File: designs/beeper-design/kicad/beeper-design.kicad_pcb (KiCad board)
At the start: 4 copper layers, 27.5 x 19.1 mm, 209 parts

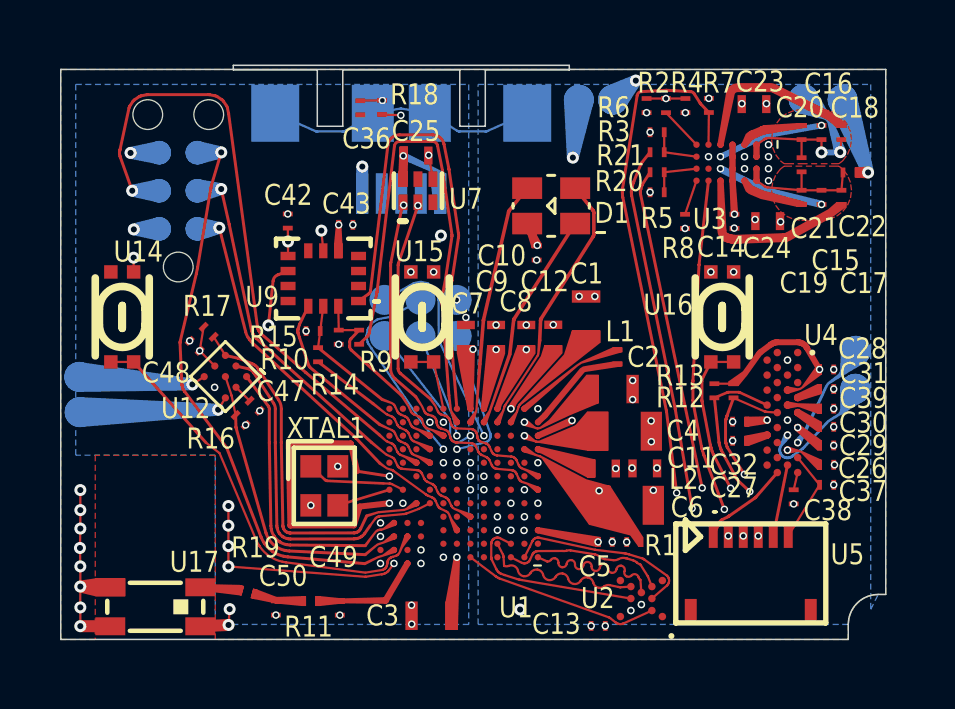
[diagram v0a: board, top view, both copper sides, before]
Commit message: latest fully routed version
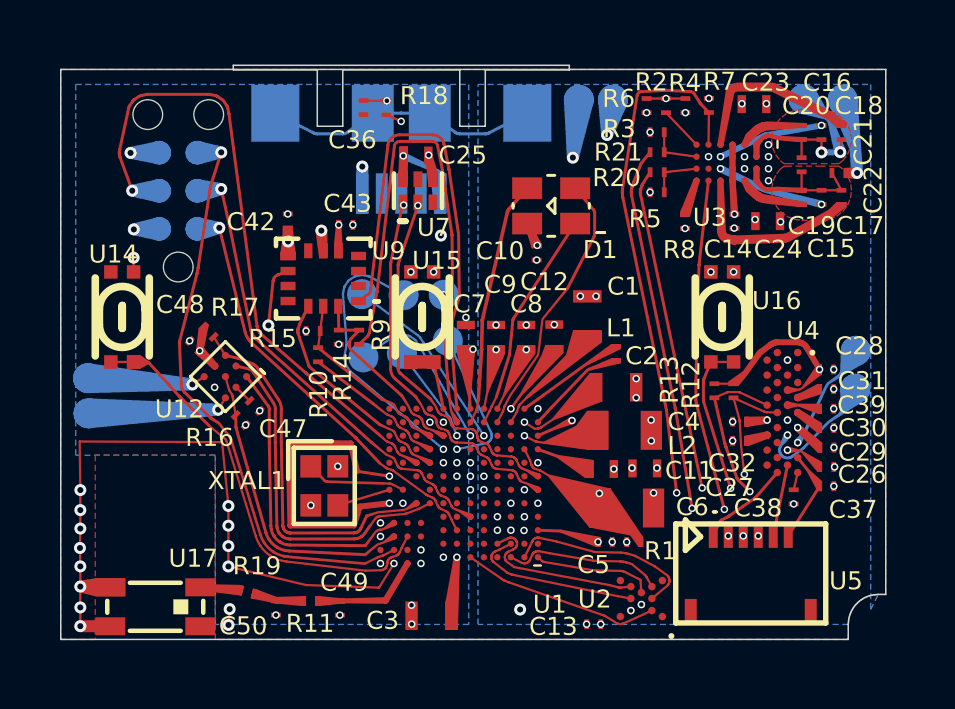
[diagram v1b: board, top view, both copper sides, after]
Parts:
- removed the ? at (143.1, 109.2)
- removed the ? at (149.4, 102.4)
- removed the ? at (141.3, 111.2)
- removed the ? at (149.9, 110.8)
- removed the ? at (151.5, 109.2)
- removed the ? at (150.7, 110.8)
- removed the ? at (149.7, 102.7)
- removed the ? at (152.1, 100.6)
- removed the ? at (148.7, 102.7)
- removed the ? at (136.6, 110.4)
- removed the ? at (148.6, 100.8)
- removed the ? at (140.2, 108.8)
- removed the C18 at (151.8, 100.6)
- removed the C2 at (144.1, 109.2)
- removed the R16 at (131.7, 110.2)
- removed the TP12 at (144.2, 99.5)
- added ?: , beeper-design:dummy114, F.Cu at (137.8, 108.2)
- added ?: , beeper-design:dummy115, F.Cu at (128.7, 102.5)
- added ?: , beeper-design:dummy117, F.Cu at (137.4, 111.5)
- added ?: , beeper-design:dummy116, F.Cu at (136.5, 110.8)
- added C28: 1u, beeper-design:Pkg0201_12, F.Cu at (151.3, 108.5)
- added C37: 1u, beeper-design:Pkg0201_10, F.Cu at (151.3, 112.4)
- added C43: 100n, beeper-design:Pkg0201_26, F.Cu at (135.3, 103.7)
- added C49: 1p, beeper-design:Pkg0201_13, F.Cu at (135.1, 116.5)
- added L2: 1u, beeper-design:Pkg0402_5, F.Cu at (143.8, 111.8)
- added R4: 20K, beeper-design:Pkg0201_34, F.Cu at (146.6, 99.7)
- added R5: 10K, beeper-design:Pkg0201_44, F.Cu at (145.6, 102.6)
- added R9: 0R, beeper-design:Pkg0201_8, F.Cu at (135.7, 107.4)
- added TP4: ~, beeper-design:SMD_TESTPT, B.Cu at (152.3, 107.9)
- added TP6: ~, beeper-design:SMD_TESTPT, B.Cu at (137.2, 106.0)
- added TP8: ~, beeper-design:SMD_TESTPT, B.Cu at (138.7, 107.5)
- added TP9: ~, beeper-design:SMD_TESTPT, B.Cu at (135.8, 108.1)
- added U15: ~, beeper-design:LP_1, F.Cu at (137.8, 106.8)
- added U16: ~, beeper-design:LP_1, F.Cu at (147.8, 106.8)
- added U17: ~, beeper-design:Pkg_2450AT18D0100_STD_R_1, F.Cu at (128.9, 116.4)
- added U2: ~, beeper-design:WLCSP_12, F.Cu at (145.1, 116.1)
- ?: renamed from U15; value ~ -> (none); footprint beeper-design:LP_2 -> beeper-design:dummy1
- ?: renamed from TP9; value ~ -> (none); footprint beeper-design:SMD_TESTPT -> beeper-design:dummy31; moved to F.Cu
- ?: renamed from R9; value 0R -> (none); footprint beeper-design:Pkg0201_32 -> beeper-design:dummy89
- ?: renamed from L2; value 1u -> (none); footprint beeper-design:Pkg0402_1 -> beeper-design:dummy17
- ?: renamed from C49; value 1p -> (none); footprint beeper-design:Pkg0201_34 -> beeper-design:dummy112
- ?: renamed from U16; value ~ -> (none); footprint beeper-design:LP_2 -> beeper-design:dummy64
- ?: renamed from R4; value 20K -> (none); footprint beeper-design:Pkg0201_18 -> beeper-design:dummy38
- ?: renamed from TP6; value ~ -> (none); footprint beeper-design:SMD_TESTPT -> beeper-design:dummy26; moved to F.Cu
- ?: renamed from C28; value 1u -> (none); footprint beeper-design:Pkg0201_19 -> beeper-design:dummy80
- ?: renamed from TP8; value ~ -> (none); footprint beeper-design:SMD_TESTPT -> beeper-design:dummy45; moved to F.Cu
- ?: renamed from U17; value ~ -> (none); footprint beeper-design:Pkg_2450AT18D0100_STD_R_1 -> beeper-design:dummy98
- ?: renamed from U2; value ~ -> (none); footprint beeper-design:WLCSP_12 -> beeper-design:dummy52
- C1: footprint beeper-design:Pkg0603_2 -> beeper-design:Pkg0603_1
- C10: footprint beeper-design:Pkg0201_8 -> beeper-design:Pkg0201_38
- C11: footprint beeper-design:Pkg0402_4 -> beeper-design:Pkg0402_7
- C12: footprint beeper-design:Pkg0402_3 -> beeper-design:Pkg0402
- C13: footprint beeper-design:Pkg0201_10 -> beeper-design:Pkg0201
- C14: footprint beeper-design:Pkg0201_1 -> beeper-design:Pkg0201_45
- C15: footprint beeper-design:Pkg0201_4 -> beeper-design:Pkg0201_42
- C16: footprint beeper-design:Pkg0201_11 -> beeper-design:Pkg0201_4
- C17: footprint beeper-design:Pkg0201_17 -> beeper-design:Pkg0201_18
- C18: renamed from C43; value 100n -> 22n; footprint beeper-design:Pkg0201_22 -> beeper-design:Pkg0201_30
- C19: renamed from TP4; value ~ -> 10n; footprint beeper-design:SMD_TESTPT -> beeper-design:Pkg0201_41; moved to F.Cu
- C2: renamed from R5; value 10K -> 22u; footprint beeper-design:Pkg0201_26 -> beeper-design:Pkg0603_2
- C20: renamed from C19; footprint beeper-design:Pkg0201_31 -> beeper-design:Pkg0201_3
- C21: footprint beeper-design:Pkg0201_46 -> beeper-design:Pkg0201_16
- C22: footprint beeper-design:Pkg0201_3 -> beeper-design:Pkg0201_28
- C23: footprint beeper-design:Pkg0402_2 -> beeper-design:Pkg0402_8
- C24: footprint beeper-design:Pkg0402_5 -> beeper-design:Pkg0402_1
- C25: footprint beeper-design:Pkg0402_6 -> beeper-design:Pkg0402_3
- C26: footprint beeper-design:Pkg0201_24 -> beeper-design:Pkg0201_7
- C27: footprint beeper-design:Pkg0201_27 -> beeper-design:Pkg0201_24
- C29: footprint beeper-design:Pkg0201_42 -> beeper-design:Pkg0201_46
- C3: footprint beeper-design:Pkg0603_1 -> beeper-design:Pkg0603
- C30: footprint beeper-design:Pkg0201_12 -> beeper-design:Pkg0201_33
- C31: footprint beeper-design:Pkg0201_16 -> beeper-design:Pkg0201_43
- C36: footprint beeper-design:Pkg0201_36 -> beeper-design:Pkg0201_2
- C38: footprint beeper-design:Pkg0201_5 -> beeper-design:Pkg0201_21
- C39: footprint beeper-design:Pkg0201_30 -> beeper-design:Pkg0201_20
- C42: footprint beeper-design:Pkg0201_15 -> beeper-design:Pkg0201_14
- C47: footprint beeper-design:Pkg0201_7 -> beeper-design:Pkg0201_27
- C48: footprint beeper-design:Pkg0201_14 -> beeper-design:Pkg0201_37
- C5: footprint beeper-design:Pkg0201_20 -> beeper-design:Pkg0201_29
- C50: footprint beeper-design:Pkg0201_44 -> beeper-design:Pkg0201_32
- C7: footprint beeper-design:Pkg0402_7 -> beeper-design:Pkg0402_2
- C8: footprint beeper-design:Pkg0402_8 -> beeper-design:Pkg0402_4
- C9: footprint beeper-design:Pkg0402 -> beeper-design:Pkg0402_6
- D1: footprint beeper-design:LP_5 -> beeper-design:LP_4
- L1: footprint beeper-design:Pkg0201_2 -> beeper-design:Pkg0201_11
- R1: footprint beeper-design:Pkg0201_43 -> beeper-design:Pkg0201_47
- R10: footprint beeper-design:Pkg0201_38 -> beeper-design:Pkg0201_17
- R11: footprint beeper-design:Pkg0201_39 -> beeper-design:Pkg0201_22
- R12, R13: footprint beeper-design:Pkg0201_9 -> beeper-design:Pkg0201_1
- R14, R15: footprint beeper-design:Pkg0201_23 -> beeper-design:Pkg0201_36
- R16: renamed from C20; value 10n -> 8K2; footprint beeper-design:Pkg0201_40 -> beeper-design:Pkg0201_5
- R17: footprint beeper-design:Pkg0201_21 -> beeper-design:Pkg0201_5
- R18: footprint beeper-design:Pkg0201_28 -> beeper-design:Pkg0201_40
- R19: footprint beeper-design:Pkg0201 -> beeper-design:Pkg0201_39
- R2: footprint beeper-design:Pkg0201_6 -> beeper-design:Pkg0201_9
- R20: footprint beeper-design:Pkg0201_29 -> beeper-design:Pkg0201_15
- R21: footprint beeper-design:Pkg0201_37 -> beeper-design:Pkg0201_25
- R3: footprint beeper-design:Pkg0201_33 -> beeper-design:Pkg0201_6
- R6: footprint beeper-design:Pkg0201_13 -> beeper-design:Pkg0201_23
- R7: footprint beeper-design:Pkg0201_41 -> beeper-design:Pkg0201_19
- R8: footprint beeper-design:Pkg0201_45 -> beeper-design:Pkg0201_31
- TP12: renamed from C37; value 1u -> ~; footprint beeper-design:Pkg0201_47 -> beeper-design:SMD_TESTPT; moved to B.Cu
- U1: footprint beeper-design:LP -> beeper-design:LP_7
- U12: footprint beeper-design:LP_7 -> beeper-design:LP_6
- U14: footprint beeper-design:LP_2 -> beeper-design:LP_1
- U3: footprint beeper-design:LP_6 -> beeper-design:LP_5
- U4: footprint beeper-design:LP_3 -> beeper-design:LP_2
- U5: footprint beeper-design:LP_4 -> beeper-design:LP_3
- U9: footprint beeper-design:LP_1 -> beeper-design:LP
- moved ? 26.2 mm to (149.8, 102.9)
- moved ? 23.9 mm to (128.3, 108.2)
- moved ? 23.4 mm to (128.2, 108.8)
- moved ? 23.2 mm to (148.7, 100.8)
- moved ? 23.1 mm to (128.7, 103.8), turned to 0 degrees
- moved R16 21.0 mm to (131.7, 110.2), turned to 45 degrees
- moved ? 20.8 mm to (143.7, 115.6)
- moved ? 20.6 mm to (146.6, 100.4)
- moved ? 20.5 mm to (147.8, 103.0)
- moved ? 20.3 mm to (148.9, 101.2)
- moved ? 20.3 mm to (149.6, 110.7)
- moved ? 19.9 mm to (128.7, 101.3)
- moved ? 19.8 mm to (134.7, 116.2)
- moved ? 19.7 mm to (152.2, 102.0)
- moved ? 19.1 mm to (151.9, 100.6)
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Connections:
- net board-io_clk renamed codec-pdm-net_clk
- net board-io_data renamed codec-pdm-net_data
- net mcu0_gpio2 renamed mcu_mcu-wpwr0_gpio
- net mcu1_gpio renamed mcu_hap-gpio1_gpio
- net mcu1_gpio2 renamed mcu_mcu-wpwr1_gpio
- net mcu2_gpio1 renamed mcu_mcu-wpwr2_gpio
- net mcu3_gpio renamed mcu_mcu-wpwr3_gpio
- net mcu_clk renamed mcu_mcu-etm_clk
- net mcu_data1 renamed mcu_mcu-etm_data1
- net mcu_scl2 renamed codec-i2c-net_scl
- net mcu_sda renamed codec-i2c-net_sda
- net mcu_sdi renamed mcu_q-spi_sdi
- ? pad trace: cap_p1 -> LZ
- ? pad trace: VBUS -> RF1 (x3)
- ? pad trace: GND -> BOOT1
- ? pad trace: mcu_sda2 -> VBUS (x2)
- ? pad trace: COMM2 -> mcu_mcu-button0_gpio
- ? pad trace: mcu_swdio -> VDD3P0 (x3)
- ? pad trace: VDD1P8P -> RECT (x3)
- ? pad trace: LX -> V18F
- ? pad trace: VBAT -> AD
- ? pad trace: VDD3P0 -> D- (x2)
- ? pad trace: VMID -> VBUS
- ? pad trace: V18F -> CLAMP1
- ? pad trace: D+ -> GND (x2)
- ? pad trace: mcu_sck -> mcu_mcu-dbg-m33_swdclk (x2)
- ? pad trace: mcu_rx -> AC2 (x3)
- ? pad trace: BOOT1 -> VBAT
- ? pad trace: COMM1 -> BOOT2
- ? pad trace: VDIG -> VDD1P8P
- ? pad trace: D- -> mcu_q-i3c_scl
- ? pad trace: board-io_r -> mcu_q-i3c_scl
- ? pad trace: RF1 -> LY
- ? pad trace: mcu0_gpio1 -> SP_N
- ? pad trace: VLED -> mcu_q-i3c_sda (x2)
- ? pad trace: mcu_tx -> VDD1P8 (x2)
- ? pad trace: V18F -> mcu_conn-uart_tx
- ? pad trace: V18F -> V14RF
- ? pad trace: mcu_sda1 -> VDDSYS (x2)
- ? pad trace: VBUS -> COMM2 (x2)
- ? pad trace: VBUS -> SP_P
- ? pad trace: FOD -> VBUS
- ? pad trace: VDD1P8 -> VMID
- ? pad trace: RF3 -> BOOT2
- ? pad trace: SP_P -> OUT-
- ? pad trace: DACREF -> GND
- ? pad trace: mcu_scl1 -> cap_p1 (x2)
- ? pad trace: LZ -> AC1
- ? pad trace: board-io_b -> VDD1P8P (x2)
- ? pad trace: mcu0_gpio -> RF2 (x2)
- ? pad trace: RF1 -> mcu_hap-gpio0_gpio (x2)
- ? pad trace: mcu_sdo -> mcu_hap-i2c_sda
- ? pad trace: RECT -> VBUS
- ? pad trace: mcu_swdclk -> AC1
- ? pad trace: VDD1P8P -> D+
- ? pad trace: V12 -> VLED (x2)
- ? pad trace: COMM1 -> mcu_hap-i2c_sda
- ? pad trace: V14RF -> mcu_q-spi_sck
- ? pad trace: GND -> OUT+
- ? pad trace: mcu_scl -> VDDSYS (x2)
- ? pad trace: GND -> V18F (x2)
- ? pad trace: RECT -> GND
- ? pad trace: VREF -> VBUS
- ? pad trace: VDD3P0 -> COMM1
- ? pad trace: board-io_g -> V12
- ? pad trace: RF2 -> FOD
- ? pad trace: mcu0_gpio1 -> mcu_q-spi_sck
- ? pad trace: mcu_swdclk -> mcu_q-spi_cs
- ? pad trace: AC2 -> DACREF
- ? pad trace: BOOT2 -> VBUS
- ? pad trace: mcu_swdclk -> mcu_q-spi_sdo
- ? pad trace: D- -> mcu_q-spi_cs
- ? pad trace: RECT -> LX
- ? pad trace: mcu_cs -> AC1
- ? pad trace: V18F -> MICBIAS1
- ? pad trace: V18F -> VDIG
- ? pad trace: V14RF -> VDD1P8 (x2)
- ? pad trace: VDD1P8 -> mcu_mcu-dbg-m33_swdclk
- ? pad trace: VBAT -> AC2
- ? pad trace: AC1 -> AC2
- ? pad trace: OUT+ -> VBAT
- ? pad trace: OUT- -> COMM1
- ? pad trace: VDDSYS -> mcu_hap-i2c_scl
- ? pad trace: RF2 -> board-io_rgb_b
- ? pad trace: VDD3P0 -> QVAR1
- ? pad trace: VBUS -> V18F
- ? pad trace: VDD1P8 -> RECT
- ? pad trace: VBAT -> VDD1P8P
- ? pad trace: AC2 -> mcu_hap-i2c_scl
- ? pad trace: COMM2 -> V14RF
- C18 pad 1: GND -> AC2
- C18 pad 2: VDD1P8 -> COMM2
- C2 pad 1: EN1 -> GND
- C2 pad 2: GND -> V14RF
- C20 pad 1: AC1 -> AC2
- C20 pad 2: BOOT1 -> BOOT2
- D1 pad 1: board-io_r -> board-io_rgb_r
- D1 pad 3: board-io_g -> board-io_rgb_g
- D1 pad 4: board-io_b -> board-io_rgb_b
- J1 pad 2: mcu_swdio -> mcu_dbg-m33_swdio
- J1 pad 3: mcu_rx -> mcu_conn-uart_rx
- J1 pad 4: mcu_swdclk -> mcu_mcu-dbg-m33_swdclk
- J1 pad 6: mcu_tx -> mcu_conn-uart_tx
- R10 pad 1: mcu_scl -> mcu_q-i3c_scl
- R10 pad 2: mcu_sck -> mcu_q-spi_sck
- R14 pad 1: mcu_sda2 -> mcu_q-i3c_sda
- R15 pad 1: mcu_scl -> mcu_q-i3c_scl
- R16 pad 1: AC2 -> mcu_hap-i2c_sda
- R16 pad 2: BOOT2 -> VDDSYS
- R17 pad 1: mcu_scl1 -> mcu_hap-i2c_scl
- U1 pad A1: mcu_sdio0 -> mcu_mcu-mem_sdio0
- U1 pad A2: mcu_sdio1 -> mcu_mcu-mem_sdio1
- U1 pad A3: mcu_sdio2 -> mcu_mcu-mem_sdio2
- U1 pad A6: mcu_cs1 -> mcu_mcu-mem_cs
- U1 pad B11: mcu_tx -> mcu_conn-uart_tx
- U1 pad B3: mcu_sdio3 -> mcu_mcu-mem_sdio3
- U1 pad B4: mcu_sck1 -> mcu_mcu-mem_sck
- U1 pad C10: mcu0_gpio1 -> mcu_mcu-button0_gpio
- U1 pad C11: mcu_sda1 -> mcu_hap-i2c_sda
- U1 pad C7: mcu_swdio -> mcu_dbg-m33_swdio
- U1 pad D11: mcu0_gpio -> mcu_hap-gpio0_gpio
- U1 pad D2: mcu2_gpio -> mcu_mcu-button2_gpio
- U1 pad D6: mcu_swdclk -> mcu_mcu-dbg-m33_swdclk
- U1 pad E10: mcu_scl1 -> mcu_hap-i2c_scl
- U1 pad H10: mcu_rx -> mcu_conn-uart_rx
- U1 pad H9: mcu_cs -> mcu_q-spi_cs
- U1 pad J7: mcu_data2 -> mcu_mcu-etm_data2
- U1 pad J8: mcu_data0 -> mcu_mcu-etm_data0
- U1 pad J9: mcu_sck -> mcu_q-spi_sck
- U1 pad K6: mcu_data3 -> mcu_mcu-etm_data3
- U1 pad K8: mcu_sda2 -> mcu_q-i3c_sda
- U1 pad K9: mcu_scl -> mcu_q-i3c_scl
- U1 pad L4: board-io_b -> board-io_rgb_b
- U1 pad L5: board-io_r -> board-io_rgb_r
- U1 pad L6: board-io_g -> board-io_rgb_g
- U1 pad L7: mcu_sdo -> mcu_q-spi_sdo
- U1 pad M8: mcu1_gpio1 -> mcu_mcu-button1_gpio
- U12 pad A1: mcu0_gpio -> mcu_hap-gpio0_gpio
- U12 pad B2: mcu_sda1 -> mcu_hap-i2c_sda
- U12 pad C1: mcu_scl1 -> mcu_hap-i2c_scl
- U14 pad A: mcu0_gpio1 -> mcu_mcu-button0_gpio
- U14 pad A1: mcu0_gpio1 -> mcu_mcu-button0_gpio
- U9 pad 12: mcu_cs -> mcu_q-spi_cs
- U9 pad 13: mcu_scl -> mcu_q-i3c_scl
- U9 pad 14: mcu_sda2 -> mcu_q-i3c_sda
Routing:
- net mcu_conn-uart_rx: track 0.00 -> 20.1 mm, vias 0 -> 1
- net mcu_rx: track 20.0 -> 0.00 mm, vias 1 -> 0
- net mcu_conn-uart_tx: track 0.00 -> 18.6 mm, vias 0 -> 1
- net mcu_tx: track 17.4 -> 0.00 mm, vias 1 -> 0
- net mcu_sdo: track 16.8 -> 0.00 mm
- net mcu_q-spi_sdo: track 0.00 -> 16.8 mm
- net mcu_mcu-button0_gpio: track 0.00 -> 13.9 mm
- net mcu_dbg-m33_swdio: track 0.00 -> 13.4 mm, vias 0 -> 1
- net mcu_mcu-dbg-m33_swdclk: track 0.00 -> 13.4 mm, vias 0 -> 1
- net mcu_swdclk: track 13.4 -> 0.00 mm, vias 1 -> 0
- net mcu0_gpio1: track 12.9 -> 0.00 mm
- net mcu2_gpio: track 12.4 -> 0.00 mm, vias 2 -> 0
- net mcu_mcu-button2_gpio: track 0.00 -> 12.4 mm, vias 0 -> 2
- net mcu_swdio: track 12.3 -> 0.00 mm, vias 1 -> 0
- net mcu_hap-i2c_scl: track 0.00 -> 11.5 mm
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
